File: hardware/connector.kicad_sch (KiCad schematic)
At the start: 5 parts, among them J1 SAFETY_SUPPLY, J2 SWDIO_CONN, J3 SENSORS, J4 VALVES, J5 MAIN

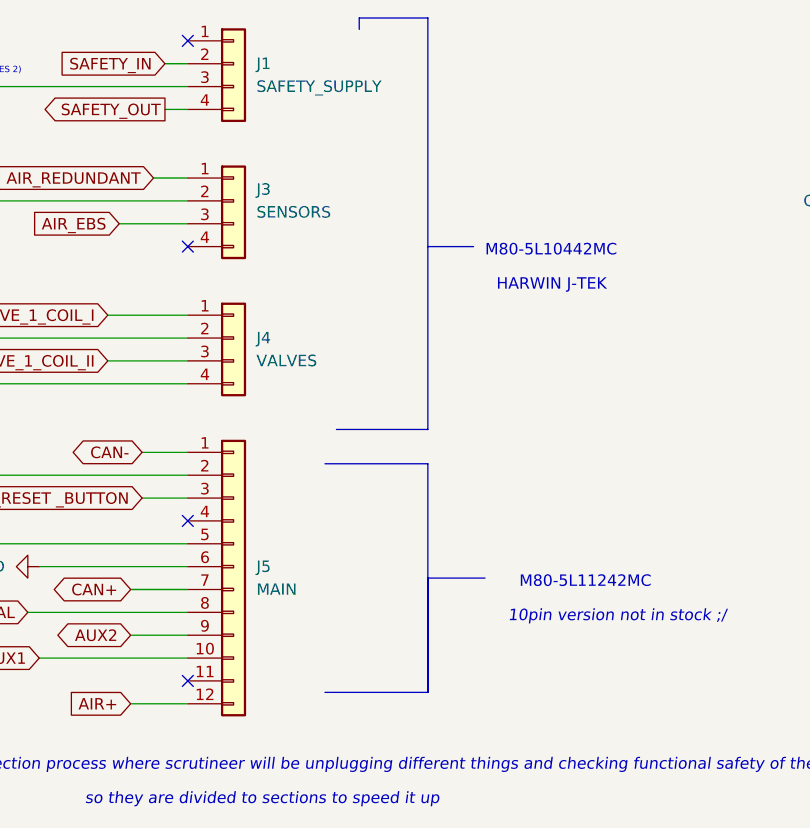
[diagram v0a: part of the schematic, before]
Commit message: uploaded older pcb version
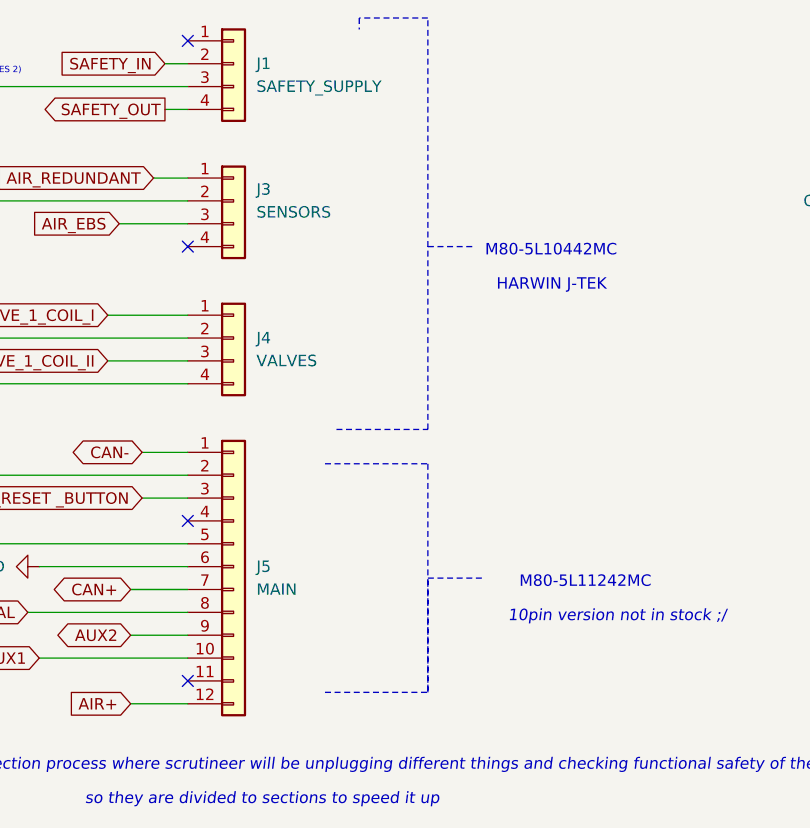
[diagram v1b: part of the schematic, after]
